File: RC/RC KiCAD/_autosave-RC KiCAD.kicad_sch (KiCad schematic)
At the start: 2 parts, among them J1 CX90B1-24P

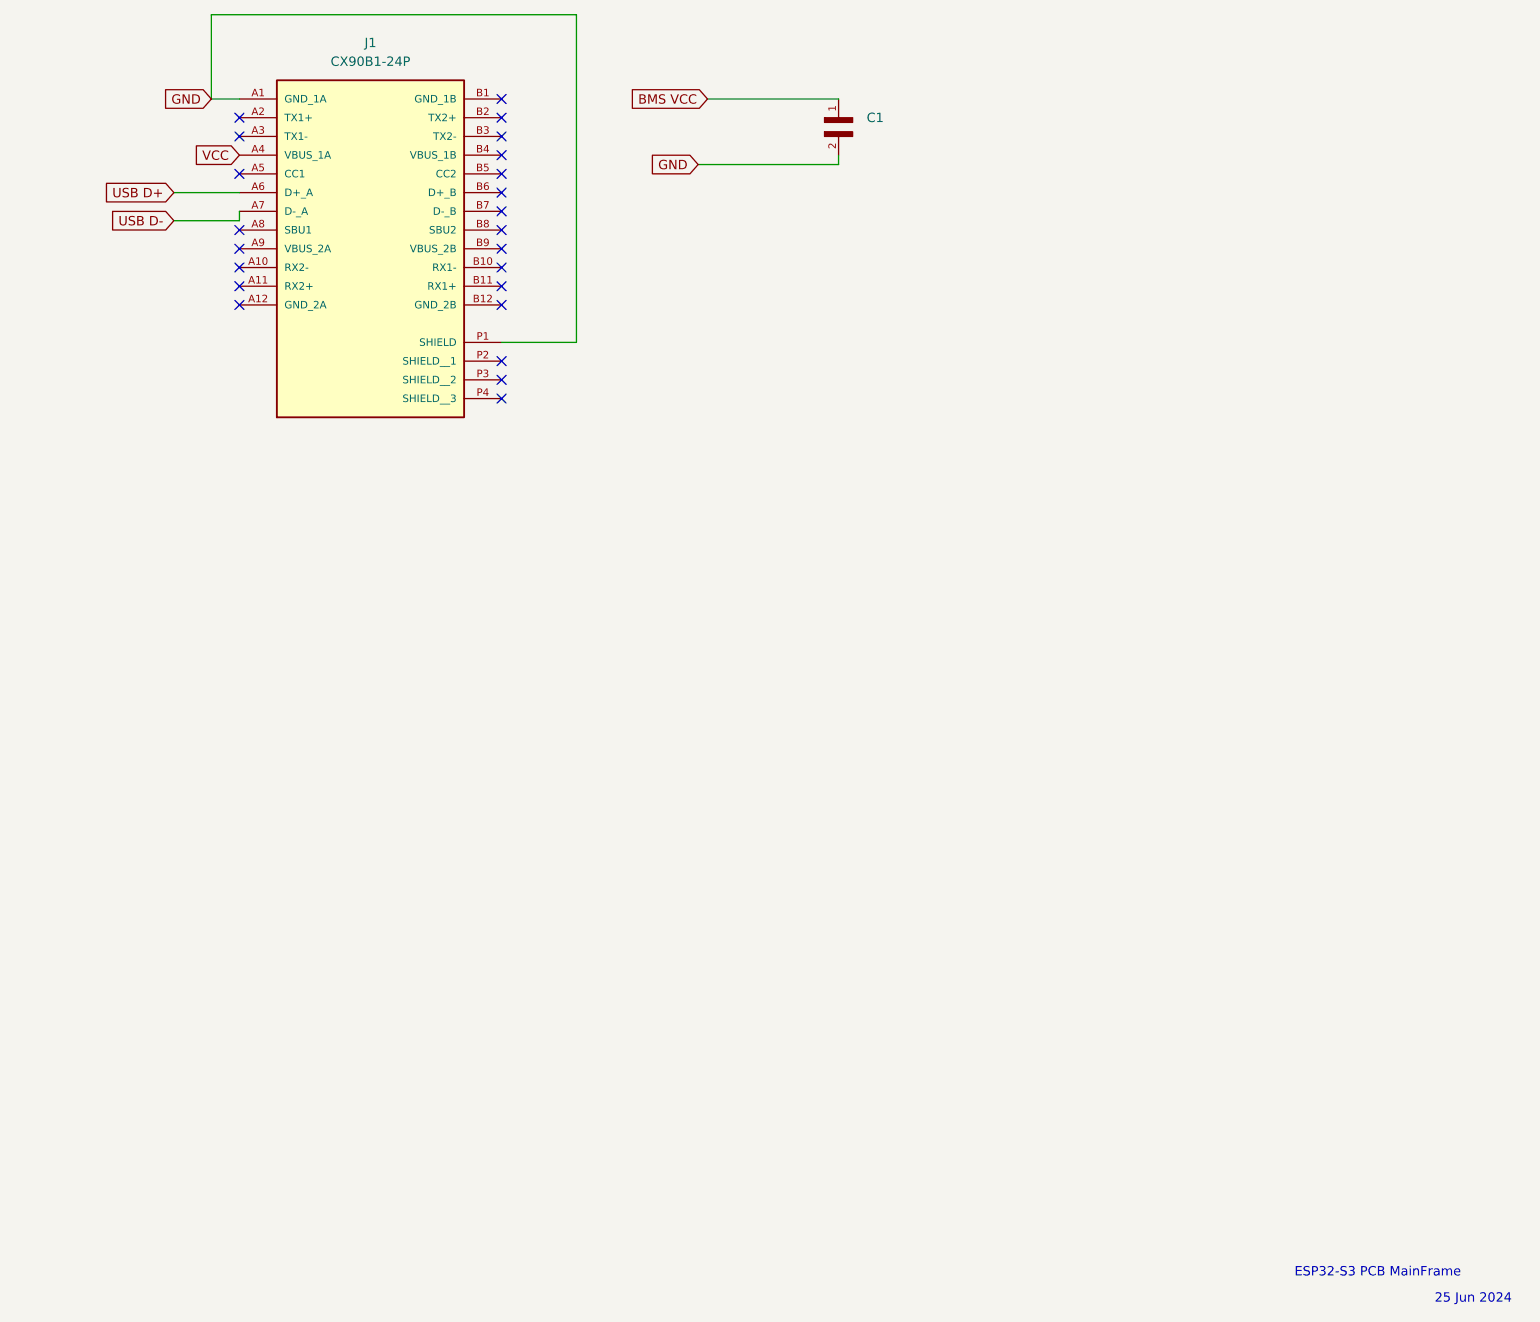
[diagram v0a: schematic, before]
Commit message: Uploading new RC PCB Components
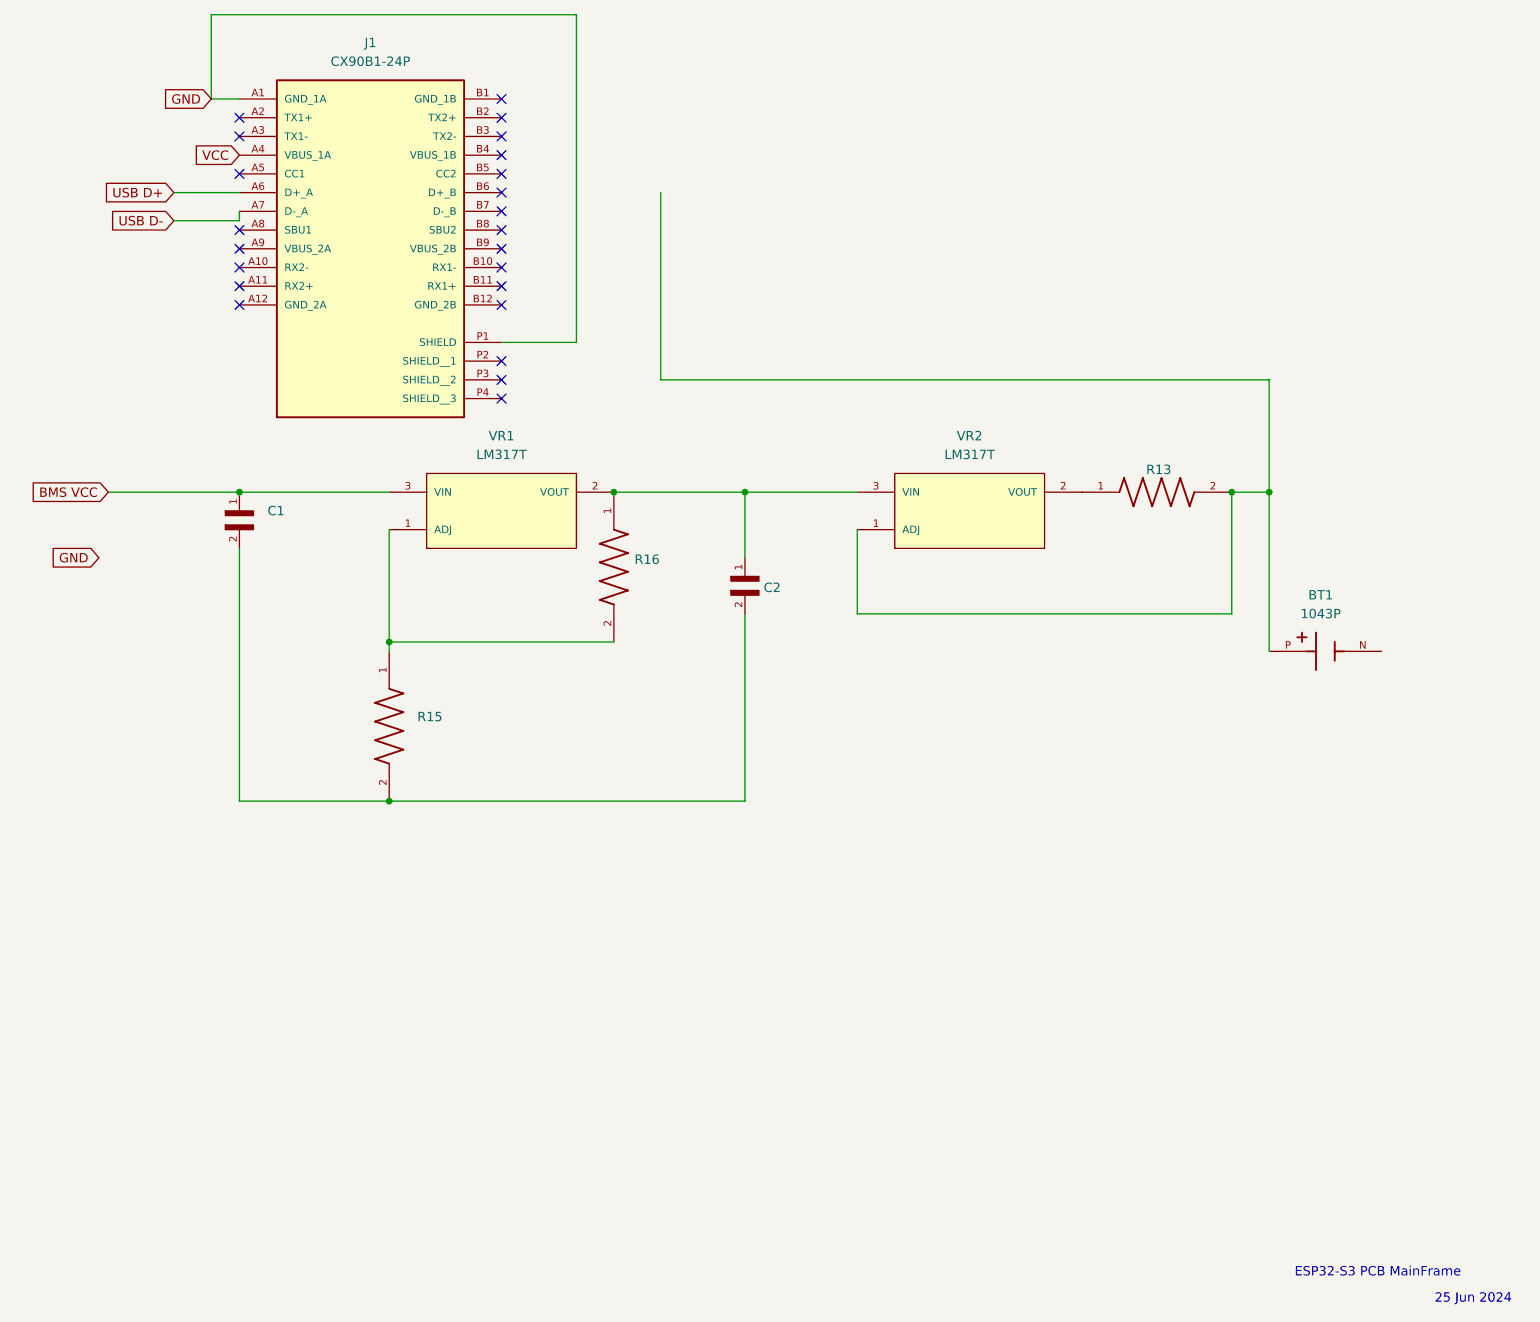
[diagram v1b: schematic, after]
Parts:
- added BT1: 1043P, 1043P:BAT_1043P, symbol 1043P:1043P
- added C2: JMK325ABJ107MM-P, JMK325ABJ107MM-P:CAPC3225X280N, symbol JMK325ABJ107MM-P:JMK325ABJ107MM-P
- added R13: CRM2512-FX-2R00ELF, CRM2512-FX-2R00ELF:RESC6331X80N, symbol CRM2512-FX-2R00ELF:CRM2512-FX-2R00ELF
- added R15: RMCF2512JT3K30, RMCF2512JT3K30:RESC6332X70N, symbol RMCF2512JT3K30:RMCF2512JT3K30
- added R16: CRCW12101K40FKEA, CRCW12101K40FKEA:RESC3225X60N, symbol CRCW12101K40FKEA:CRCW12101K40FKEA
- added VR1, VR2: LM317T, LM317T:TO254P1054X470X1955-3, symbol LM317T:LM317T
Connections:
- net BMS VCC: now also VR1.3 (VIN)
- net GND: no longer C1.2
- new net: C2.1, R16.1, VR1.2 (VOUT), VR2.3 (VIN)
- new net: R15.1, R16.2, VR1.1 (ADJ)
- new net: C1.2, C2.2, R15.2
- new net: BT1.P, R13.2, VR2.1 (ADJ)
- new net: R13.1, VR2.2 (VOUT)
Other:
- moved on the sheet: C1
